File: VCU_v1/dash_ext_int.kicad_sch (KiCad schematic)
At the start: 55 parts, among them Q3 SP8K80TB1, Q4 SP8K80TB1, Q5 SP8K80TB1

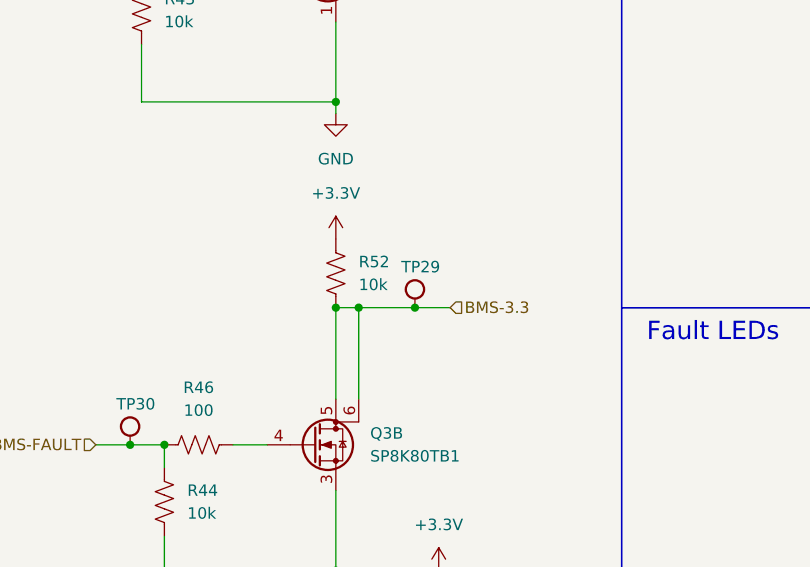
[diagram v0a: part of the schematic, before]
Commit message: begin pcb design
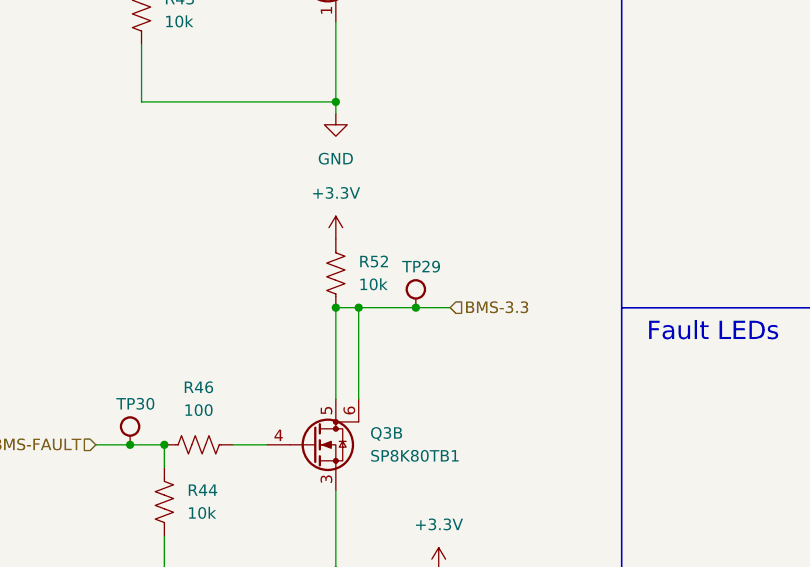
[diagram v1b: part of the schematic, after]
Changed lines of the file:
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@@
 	)
 	(junction
-		(at 64.6693 87.63)
-		(diameter 0)
-		(color 0 0 0 0)
-	)
-	(junction
 		(at 125.73 102.87)
 		(diameter 0)
@@
 	)
 	(junction
+		(at 64.77 87.63)
+		(diameter 0)
+		(color 0 0 0 0)
+	)
+	(junction
 		(at 67.31 124.46)
 		(diameter 0)
@@
 	(wire
 		(pts
-			(xy 58.42 87.63) (xy 64.6693 87.63)
+			(xy 58.42 87.63) (xy 64.77 87.63)
 		)
 		(stroke
@@
 	(wire
 		(pts
+			(xy 64.77 87.63) (xy 68.58 87.63)
+		)
+		(stroke
+			(width 0)
+			(type default)
+		)
+	)
+	(wire
+		(pts
 			(xy 168.91 69.85) (xy 168.91 73.66)
 		)
@@
 	(wire
 		(pts
-			(xy 64.6693 87.63) (xy 68.58 87.63)
-		)
-		(stroke
-			(width 0)
-			(type default)
-		)
-	)
-	(wire
-		(pts
 			(xy 163.83 130.81) (xy 163.83 138.43)
 		)
@@
 	(symbol
 		(lib_id ".Test-Point:RH-5015")
-		(at 64.6693 87.63 0)
+		(at 64.77 87.63 0)
 		(unit 1)
 		(exclude_from_sim no)
@@
 		(dnp no)
 		(property "Reference" "TP29"
-			(at 63.1461 82.3737 0)
+			(at 63.2468 82.3737 0)
 			(effects
 				(font
@@
 		)
 		(property "Value" "RH-5015"
-			(at 63.1461 80.2235 0)
+			(at 63.2468 80.2235 0)
 			(effects
 				(font
@@
 		)
 		(property "Footprint" "TestPoint:TestPoint_Keystone_5015_Micro_Mini"
-			(at 64.6693 99.06 0)
+			(at 64.77 99.06 0)
 			(effects
 				(font
@@
 		)
 		(property "Datasheet" "https://wmsc.lcsc.com/wmsc/upload/file/pdf/v2/lcsc/2310260935_ronghe-RH-5015_C5199798.pdf"
-			(at 64.6693 102.87 0)
+			(at 64.77 102.87 0)
 			(effects
 				(font
@@
 		)
 		(property "Description" "Surface-mount grabby test point"
-			(at 64.6693 106.68 0)
+			(at 64.77 106.68 0)
 			(effects
 				(font
@@
 		)
 		(property "Link" "https://jlcpcb.com/partdetail/Ronghe-RH5015/C5199798"
-			(at 64.6693 110.49 0)
+			(at 64.77 110.49 0)
 			(effects
 				(font
@@
 		)
 		(property "Digikey P/N" "36-5015CT-ND"
-			(at 64.6693 121.92 0)
+			(at 64.77 121.92 0)
 			(effects
 				(font
@@
 		)
 		(property "Mouser P/N" "534-5015"
-			(at 64.6693 125.73 0)
+			(at 64.77 125.73 0)
 			(effects
 				(font
@@
 		)
 		(property "LCSC P/N" "C5199798"
-			(at 64.6693 129.54 0)
+			(at 64.77 129.54 0)
 			(effects
 				(font
@@
 		)
 		(property "Manufacturer" "Ronghe"
-			(at 64.6693 114.3 0)
+			(at 64.77 114.3 0)
 			(effects
 				(font
@@
 		)
 		(property "Manufacturer P/N" "RH-5015"
-			(at 64.6693 118.11 0)
+			(at 64.77 118.11 0)
 			(effects
 				(font
@@
 		)
 		(property "LCSC Part #" "C5199798"
-			(at 64.6693 87.63 0)
+			(at 64.77 87.63 0)
 			(effects
 				(font
